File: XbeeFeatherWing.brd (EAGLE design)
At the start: 124.5 x 67.3 mm, 18 parts

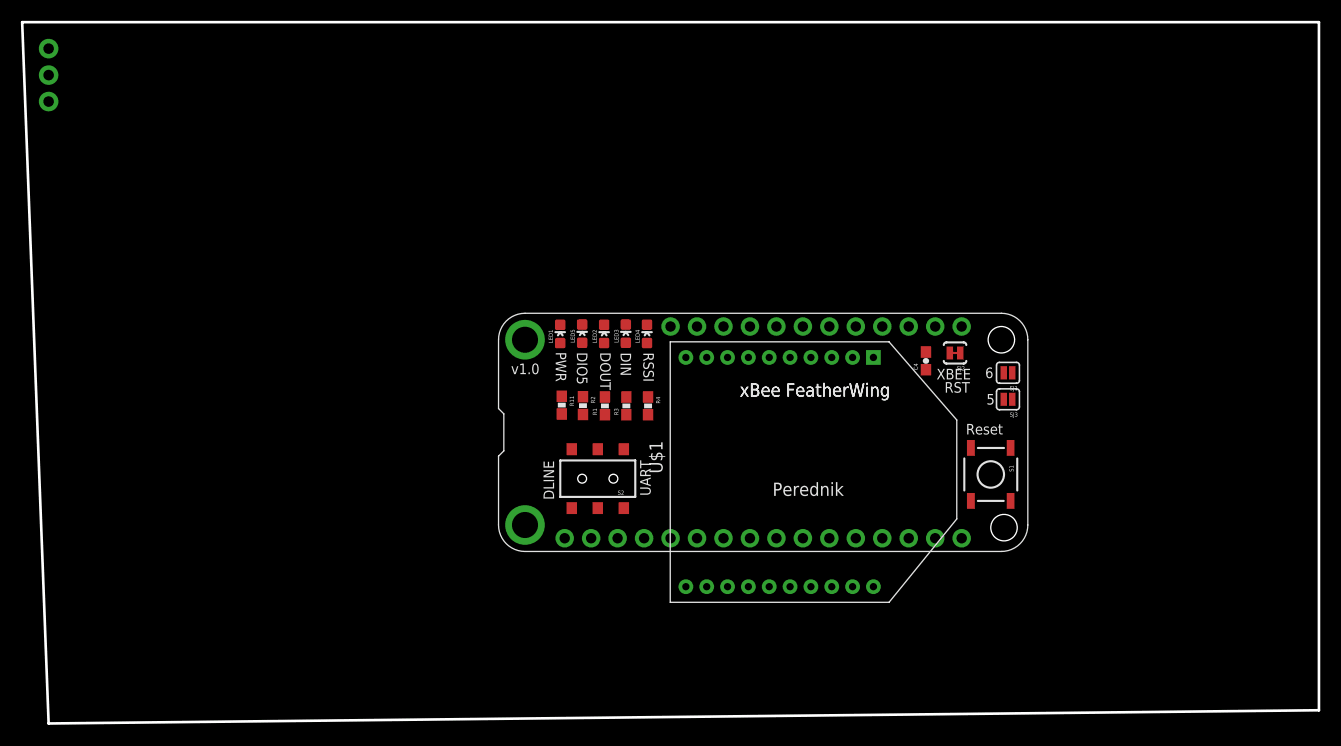
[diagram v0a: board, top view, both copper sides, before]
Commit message: routing complete
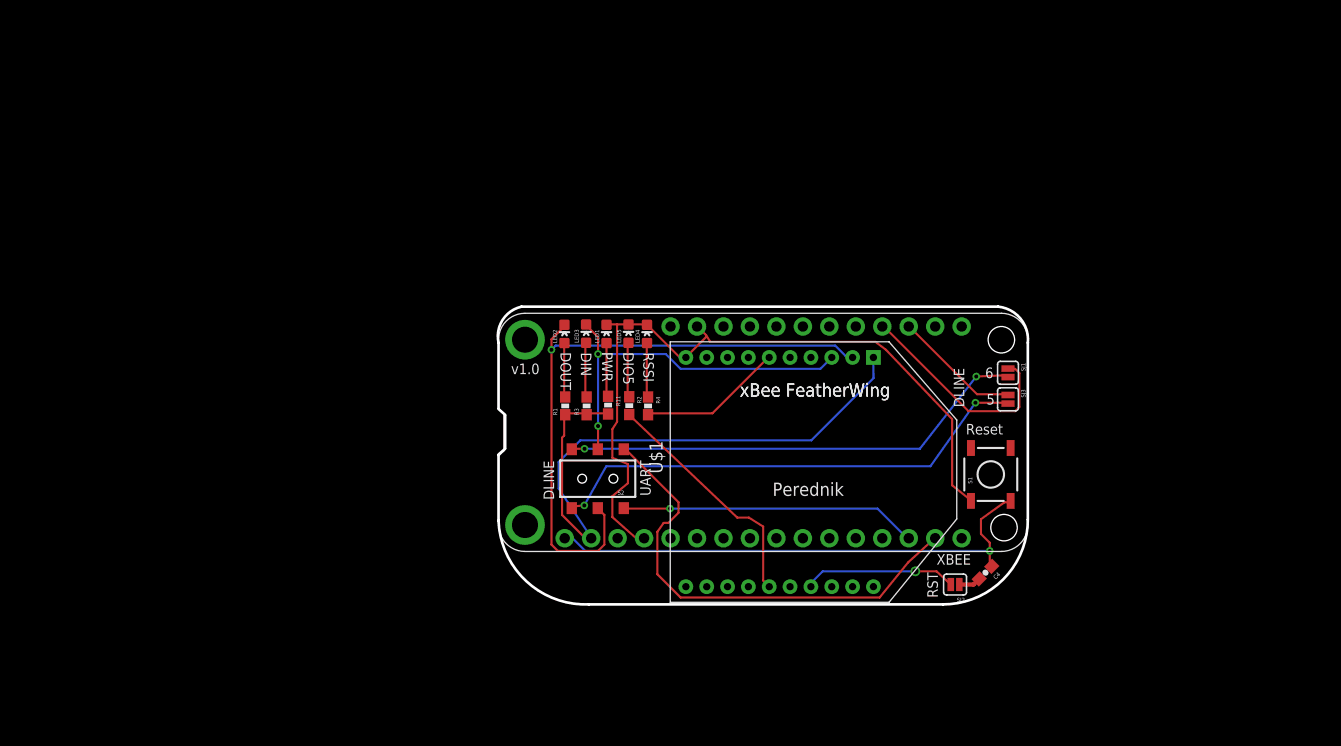
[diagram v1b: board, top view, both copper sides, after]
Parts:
- SJ2: value SOLDERJUMPERTRACE -> SOLDERJUMPERNC; device SparkFun:SJ_2S-TRACE -> SparkFun-Retired:SJ_2S
- moved SJ2 22.2 mm to (89.5, 5.71)
- moved C4 21.1 mm to (92.5, 6.86), turned to 225 degrees
- moved LED1 4.45 mm to (56.1, 29.8)
- moved LED5 4.45 mm to (58.2, 29.8)
- moved R11 4.45 mm to (56.2, 22.9)
- moved R2 4.45 mm to (58.3, 22.9)
- moved R3 3.81 mm to (54.2, 22.9)
- moved LED2 3.81 mm to (52.0, 29.8)
- moved LED3 3.81 mm to (54.1, 29.8)
- moved R1 3.81 mm to (52.1, 22.9)
- turned S1 to 90 degrees
- turned SJ1 to 270 degrees
- turned SJ3 to 270 degrees
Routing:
- net GND: track 0.00 -> 73.1 mm
- net 3.3V: track 0.00 -> 61.7 mm
- net DOUT: track 0.00 -> 60.5 mm, vias 0 -> 1
- net RST: track 0.00 -> 49.7 mm, vias 0 -> 1
- net N$141: track 0.00 -> 47.3 mm, vias 0 -> 2
- net UART_TX: track 0.00 -> 45.4 mm
- net N$140: track 0.00 -> 45.4 mm, vias 0 -> 2
- net DIN: track 0.00 -> 35.9 mm, vias 0 -> 2
- net UART_RX: track 0.00 -> 28.5 mm, vias 0 -> 1
- net DIO5: track 0.00 -> 23.1 mm
- net D_TX: track 0.00 -> 21.2 mm
- net DIO3: track 0.00 -> 14.7 mm, vias 0 -> 1
- net RSSI: track 0.00 -> 13.9 mm
- net D_RX: track 0.00 -> 12.2 mm
- net N$139: track 0.00 -> 5.34 mm
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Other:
- board size 124.5 x 67.3 mm -> 50.9 x 28.6 mm
